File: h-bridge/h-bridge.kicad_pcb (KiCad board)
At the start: 2 copper layers, 67.9 x 50.5 mm, 27 parts, among them J1 Screw_Terminal_01x06, Q1 2N2222, Q2 IRF4905, Q3 IRLZ44N, Q4 IRF4905, Q5 IRF4905, Q6 IRF4905, Q7 IRLZ44N, Q8 2N2222

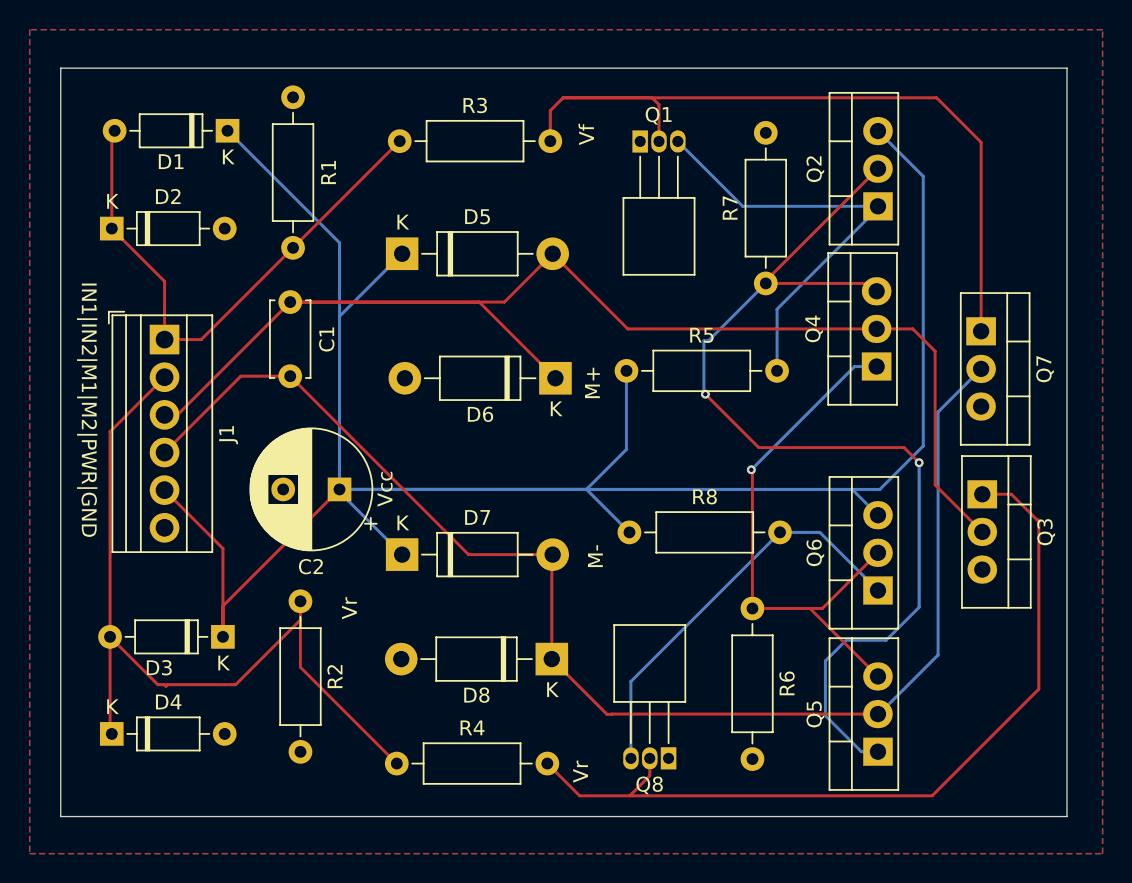
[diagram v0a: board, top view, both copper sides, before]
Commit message: V3 submitted to JLCPCB
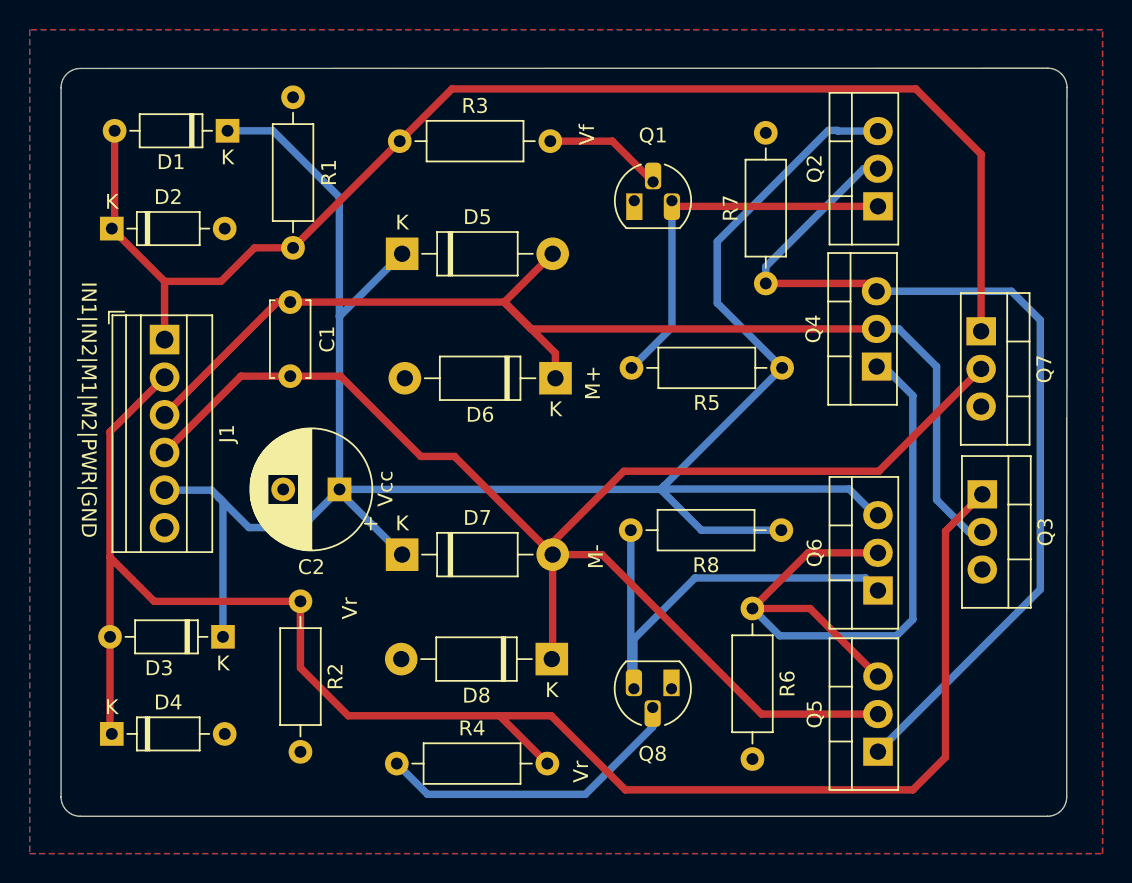
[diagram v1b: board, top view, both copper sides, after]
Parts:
- Q1, Q8: footprint Package_TO_SOT_THT:TO-92_Inline_Horizontal1 -> Package_TO_SOT_THT:TO-92_HandSolder
- Q2, Q4, Q5, Q6: value IRF4905 -> FQP27P06
- moved R5 10.5 mm to (143.6, 89.2), turned to 180 degrees
- moved R8 10.3 mm to (143.5, 100.2), turned to 180 degrees
- moved Q8 4.70 mm to (136.1, 110.9)
- moved Q1 4.02 mm to (133.6, 77.9)
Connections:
- D1 pad 2: Net-(D1-A) -> Vf
- D2 pad 1: Net-(D1-A) -> Vf
- D3 pad 2: Net-(D3-A) -> Vr
- D4 pad 1: Net-(D3-A) -> Vr
- J1 pad 1: Net-(D1-A) -> Vf
- J1 pad 2: Net-(D3-A) -> Vr
- Q1 pad 2: Vf -> Net-(Q1-B)
- Q8 pad 2: Vr -> Net-(Q8-B)
- R1 pad 1: Net-(D1-A) -> Vf
- R2 pad 1: Net-(D3-A) -> Vr
- R3 pad 1: Net-(D1-A) -> Vf
- R3 pad 2: Vf -> Net-(Q1-B)
- R4 pad 1: Net-(D3-A) -> Net-(Q8-B)
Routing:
- net Vr: track 56.1 -> 115.4 mm
- net Vcc: track 205.9 -> 146.8 mm
- net Net-(D3-A): track 56.6 -> 0.00 mm
- net Net-(D1-A): track 37.1 -> 0.00 mm
- net Vf: track 54.6 -> 89.9 mm
- net Net-(Q8-B): track 0.00 -> 21.3 mm
- net M+: track 92.8 -> 81.0 mm
- net M-: track 90.2 -> 101.4 mm
- net Net-(Q4-G): track 41.1 -> 50.8 mm, vias 1 -> 0
- net Net-(Q1-B): track 0.00 -> 8.07 mm
- net Net-(Q2-D): track 70.2 -> 64.7 mm, vias 2 -> 0
- net Net-(Q6-G): track 27.7 -> 32.7 mm
- net Net-(Q1-C): track 29.2 -> 26.5 mm
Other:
- outline, holes or cut-outs redrawn
